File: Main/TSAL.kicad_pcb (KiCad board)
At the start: 2 copper layers, 140 x 70 mm, 156 parts, among them J1 Micro-Fit, J2 Mini-SPOX, J3 Mini-SPOX, J4 Mini-SPOX, J5 Mini-SPOX, Q1 IRLML2502, Q10 NPN, Q11 MJD122, Q12 PNP, Q2 IRLML2502, Q3 IRLML2502, Q4 IRLML2502, Q5 IRLML2502, Q6 BSC0904NSI, Q7 BSC0902NSI, Q8 BSC0902NSI, Q9 MJD122, U1 74HC08, U10 TLV431, U11 TLV431, U2 74HC08, U3 LMC555, U4 TPS562200, U5 TPS63020, U6 MAX40200AUK, U7 INA180A3, U8 TLV9104, U9 LM25117

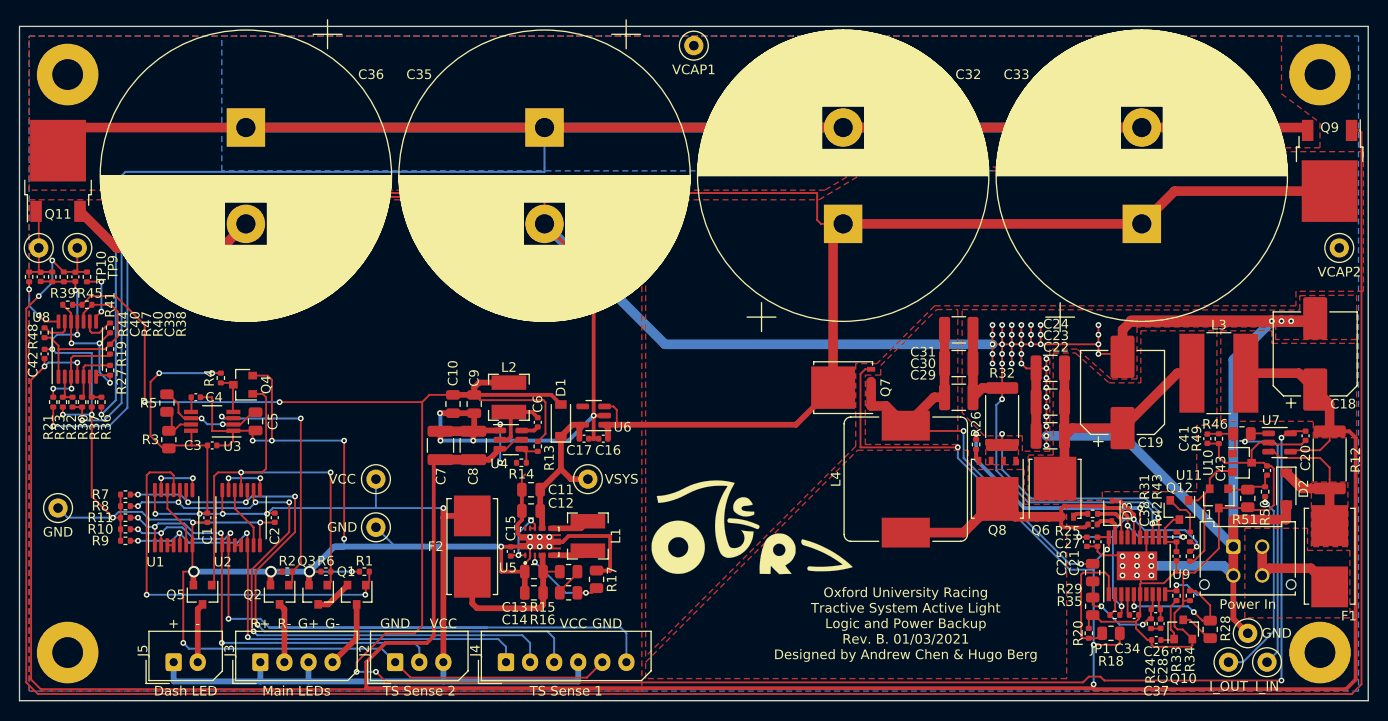
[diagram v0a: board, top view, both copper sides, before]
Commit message: hv sense v2
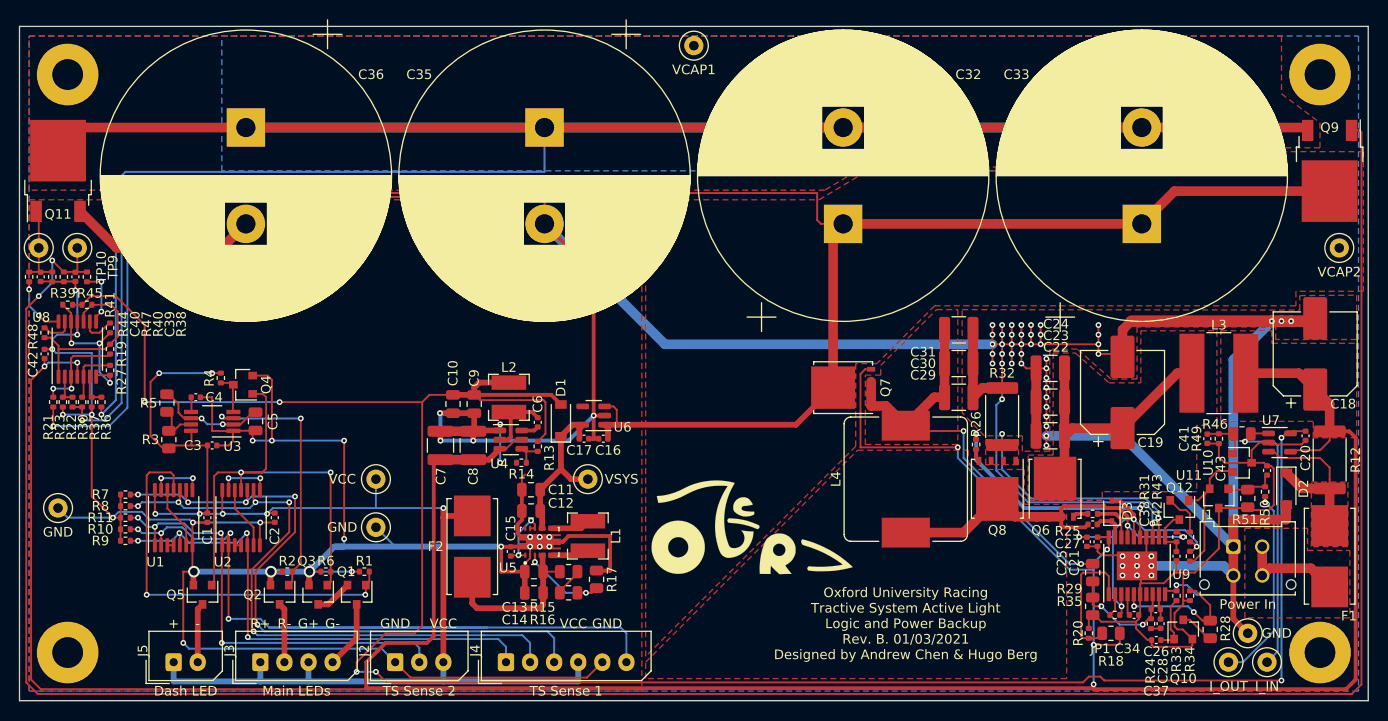
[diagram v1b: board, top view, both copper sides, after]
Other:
- net class Default removed
